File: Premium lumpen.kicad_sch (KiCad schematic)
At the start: 148 parts, among them J1 Conn_01x04_MountingPin, J2 AVR-ISP-6, SW1 SW_Push, SW2 RotaryEncoder_Switch, SW3 RotaryEncoder_Switch, SW4 RotaryEncoder_Switch, SW5 RotaryEncoder_Switch, U1 ATmega32U4-M, Y1 Crystal_GND24_Small

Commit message: premium 3 flex cut matrix routed
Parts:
- Drgb1, Drgb10, Drgb11, Drgb12, Drgb13, Drgb14, Drgb15, Drgb16, Drgb17, Drgb18, Drgb19, Drgb2, Drgb20, Drgb21, Drgb22, Drgb23, Drgb24, Drgb25, Drgb26, Drgb27, Drgb28, Drgb29, Drgb3, Drgb30, Drgb31, Drgb32, Drgb33, Drgb34, Drgb35, Drgb36, Drgb37, Drgb38, Drgb39, Drgb4, Drgb40, Drgb41, Drgb42, Drgb43, Drgb44, Drgb45, Drgb46, Drgb47, Drgb48, Drgb49, Drgb50, Drgb51, Drgb7, Drgb8, Drgb9: footprint Keebio-Parts:SK6812-MINI-E -> CrumpPrints:WS2812-2020

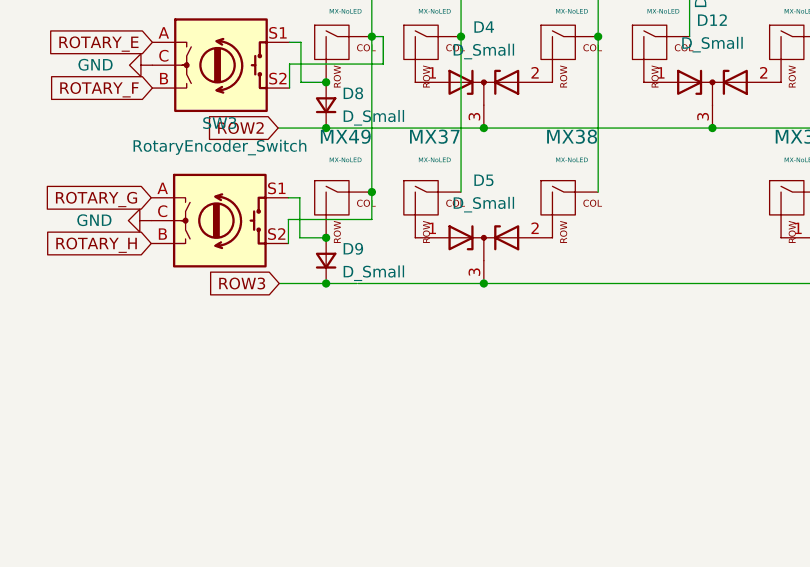
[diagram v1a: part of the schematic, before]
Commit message: auto save
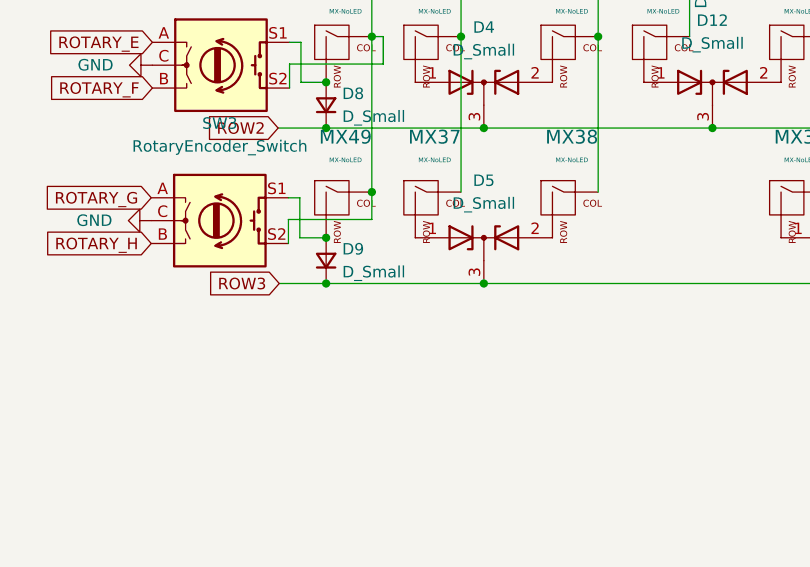
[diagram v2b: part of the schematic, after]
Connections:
- net  ROW3: now also D16.3 (K), D24.1 (K), D31.3 (K), D42.3 (K), D5.3 (K)
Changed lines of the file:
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@@
   (junction (at 238.125 109.982) (diameter 0) (color 0 0 0 0)
   )
+  (junction (at 149.225 109.982) (diameter 0) (color 0 0 0 0)
+  )
   (junction (at 200.025 57.15) (diameter 0) (color 0 0 0 0)
   )
@@
   )
   (junction (at 381.381 102.235) (diameter 0) (color 0 0 0 0)
-  )
-  (junction (at 149.225 109.982) (diameter 0) (color 0 0 0 0)
   )
   (junction (at 250.825 74.93) (diameter 0) (color 0 0 0 0)
@@
     (stroke (width 0) (type default) (color 0 0 0 0))
   )
-  (wire (pts (xy 135.255 109.982) (xy 149.225 109.982))
-    (stroke (width 0) (type default) (color 0 0 0 0))
-  )
   (wire (pts (xy 50.546 28.321) (xy 50.546 30.861))
     (stroke (width 0) (type default) (color 0 0 0 0))
@@
     (stroke (width 0) (type default) (color 0 0 0 0))
   )
-  (wire (pts (xy 131.699 109.982) (xy 135.128 109.982))
+  (wire (pts (xy 131.699 109.982) (xy 149.225 109.982))
     (stroke (width 0) (type default) (color 0 0 0 0))
   )
@@
     (stroke (width 0) (type default) (color 0 0 0 0))
   )
+  (wire (pts (xy 149.225 109.982) (xy 189.865 109.982))
+    (stroke (width 0) (type default) (color 0 0 0 0))
+  )
   (wire (pts (xy 138.049 64.77) (xy 136.779 64.77))
     (stroke (width 0) (type default) (color 0 0 0 0))
@@
     (stroke (width 0) (type default) (color 0 0 0 0))
   )
-  (wire (pts (xy 149.225 109.982) (xy 189.865 109.982))
-    (stroke (width 0) (type default) (color 0 0 0 0))
-  )

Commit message: premium work
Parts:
- Drgb1, Drgb10, Drgb11, Drgb12, Drgb13, Drgb14, Drgb15, Drgb16, Drgb17, Drgb18, Drgb19, Drgb2, Drgb20, Drgb21, Drgb22, Drgb23, Drgb24, Drgb25, Drgb26, Drgb27, Drgb28, Drgb29, Drgb3, Drgb30, Drgb31, Drgb32, Drgb33, Drgb34, Drgb35, Drgb36, Drgb37, Drgb38, Drgb39, Drgb4, Drgb40, Drgb41, Drgb42, Drgb43, Drgb44, Drgb45, Drgb46, Drgb47, Drgb48, Drgb49, Drgb50, Drgb51, Drgb7, Drgb8, Drgb9: footprint CrumpPrints:WS2812-2020 -> Keebio-Parts:SK6812-MINI-E
